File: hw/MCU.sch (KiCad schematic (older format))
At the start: 1 part, among them U11 EFM32HG310F64G-B-QFN32

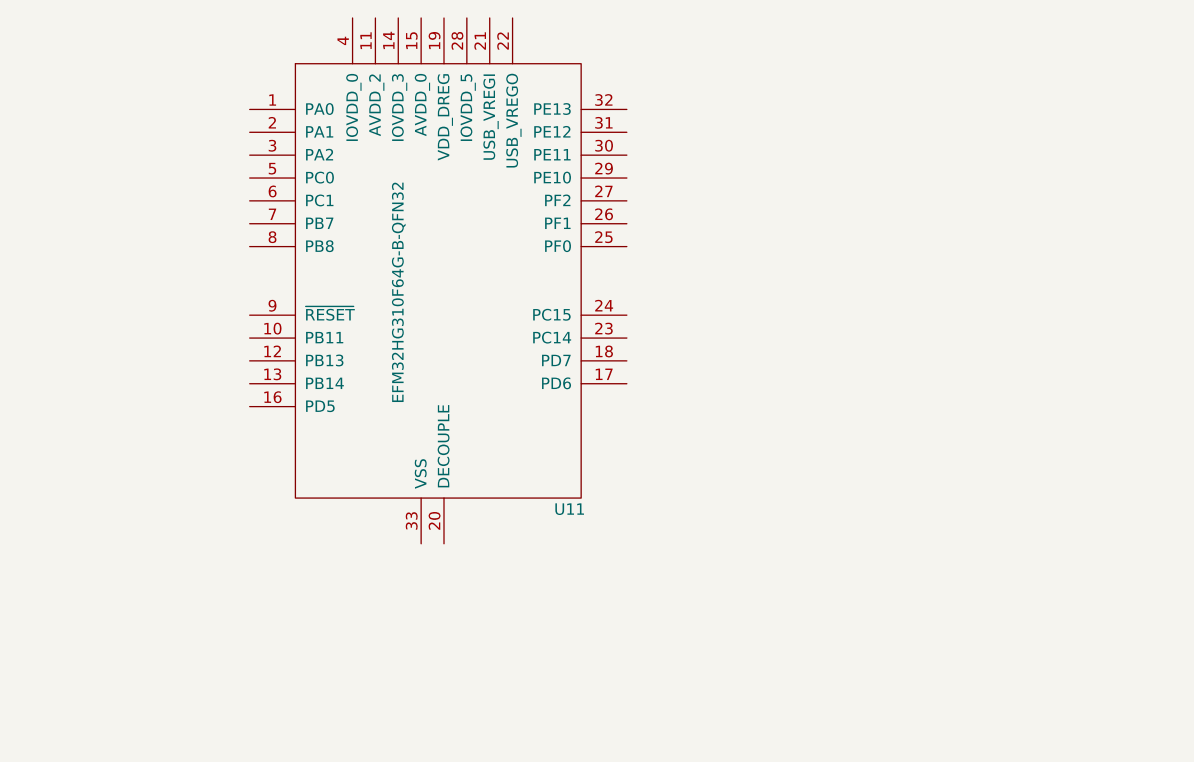
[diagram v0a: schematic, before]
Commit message: minor fixes
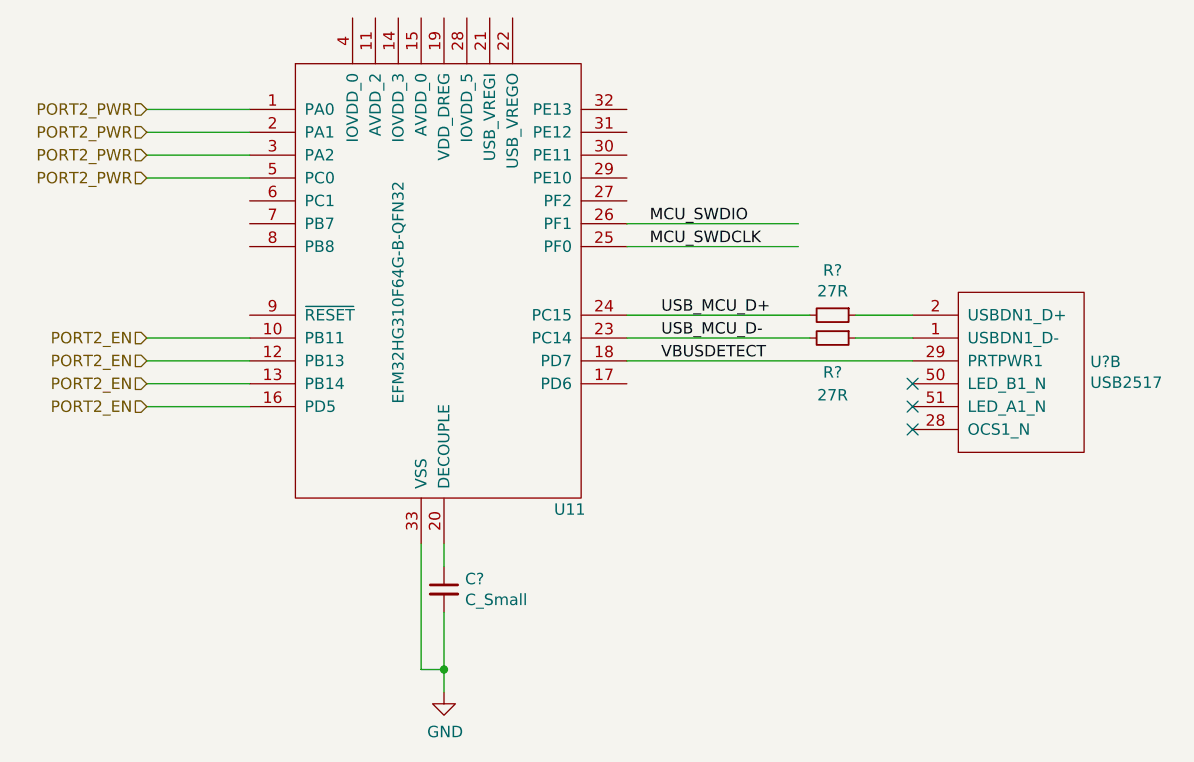
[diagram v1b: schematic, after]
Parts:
- added C?: C_Small, symbol Device:C_Small
- added R? (x2): 27R, symbol Device:R_Small
- added U?: USB2517, symbol USB2517:USB2517
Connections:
- net labels added: GND, MCU_SWDCLK, MCU_SWDIO, PORT2_EN, PORT2_PWR, USB_MCU_D+, USB_MCU_D-, VBUSDETECT
- wire segments 0 -> 20
- no-connect marks 0 -> 3
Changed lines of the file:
@@
 	1    0    0    -1
 $EndComp
+$Comp
+L power:GND #PWR?
+U 1 1 5BB092EA
+P 4650 5050
+F 0 "#PWR?" H 4650 4800 50  0001 C CNN
+F 1 "GND" H 4655 4877 50  0000 C CNN
+F 2 "" H 4650 5050 50  0001 C CNN
+F 3 "" H 4650 5050 50  0001 C CNN
+	1    4650 5050
+	1    0    0    -1
+$EndComp
+Wire Wire Line
+	4550 4400 4550 4950
+Wire Wire Line
+	4550 4950 4650 4950
+Wire Wire Line
+	4650 4950 4650 5050
+$Comp
+L USB2517:USB2517 U?
+U 2 1 5BB8A495
+P 7150 3650
+F 0 "U?" H 6823 3604 50  0000 R CNN
+F 1 "USB2517" H 6823 3695 50  0000 R CNN
+F 2 "" H 8250 5450 50  0001 C CNN
+F 3 "" H 8250 5450 50  0001 C CNN
+	2    7150 3650
+	-1   0    0    1
+$EndComp
+Text Label 5600 3400 0    50   ~ 0
+USB_MCU_D+
+Text Label 5600 3500 0    50   ~ 0
+USB_MCU_D-
+NoConn ~ 6700 3700
+NoConn ~ 6700 3800
+NoConn ~ 6700 3900
+Wire Wire Line
+	5450 3000 6200 3000
+Wire Wire Line
+	5450 3100 6200 3100
+Text Label 5550 3000 0    50   ~ 0
+MCU_SWDIO
+Text Label 5550 3100 0    50   ~ 0
+MCU_SWDCLK
+Wire Wire Line
+	6700 3600 5450 3600
+Text Label 5600 3600 0    50   ~ 0
+VBUSDETECT
+Text HLabel 3350 2500 0    50   Input ~ 0
+PORT2_PWR
+Text HLabel 3350 2600 0    50   Input ~ 0
+PORT2_PWR
+Text HLabel 3350 2700 0    50   Input ~ 0
+PORT2_PWR
+Text HLabel 3350 2800 0    50   Input ~ 0
+PORT2_PWR
+Text HLabel 3350 3500 0    50   Input ~ 0
+PORT2_EN
+Text HLabel 3350 3600 0    50   Input ~ 0
+PORT2_EN
+Text HLabel 3350 3700 0    50   Input ~ 0
+PORT2_EN
+Text HLabel 3350 3800 0    50   Input ~ 0
+PORT2_EN
+Wire Wire Line
+	3800 3500 3350 3500
+Wire Wire Line
+	3350 3600 3800 3600
+Wire Wire Line
+	3800 3700 3350 3700
+Wire Wire Line
+	3800 3800 3350 3800
+Wire Wire Line
+	3350 2500 3800 2500
+Wire Wire Line
+	3350 2600 3800 2600
+Wire Wire Line
+	3350 2700 3800 2700
+Wire Wire Line
+	3800 2800 3350 2800
+$Comp
+L Device:C_Small C?
+U 1 1 5BC29C29
+P 4650 4600
+F 0 "C?" H 4742 4646 50  0000 L CNN
+F 1 "C_Small" H 4742 4555 50  0000 L CNN
+F 2 "" H 4650 4600 50  0001 C CNN
+F 3 "~" H 4650 4600 50  0001 C CNN
+	1    4650 4600
+	1    0    0    -1
+$EndComp
+Wire Wire Line
+	4650 4400 4650 4500
+Wire Wire Line
+	4650 4700 4650 4950
+Connection ~ 4650 4950
+$Comp
+L Device:R_Small R?
+U 1 1 5BC2A861
+P 6350 3400
+F 0 "R?" V 6154 3400 50  0000 C CNN
+F 1 "27R" V 6245 3400 50  0000 C CNN
+F 2 "" H 6350 3400 50  0001 C CNN
+F 3 "~" H 6350 3400 50  0001 C CNN
+	1    6350 3400
+	0    1    1    0
+$EndComp
+$Comp
+L Device:R_Small R?
+U 1 1 5BC2A890
+P 6350 3500
+F 0 "R?" V 6500 3500 50  0000 C CNN
+F 1 "27R" V 6600 3500 50  0000 C CNN
+F 2 "" H 6350 3500 50  0001 C CNN
+F 3 "~" H 6350 3500 50  0001 C CNN
+	1    6350 3500
+	0    1    1    0
+$EndComp
+Wire Wire Line
+	6700 3400 6450 3400
+Wire Wire Line
+	6700 3500 6450 3500
+Wire Wire Line
+	6250 3500 5450 3500
+Wire Wire Line
+	6250 3400 5450 3400
 $EndSCHEMATC
